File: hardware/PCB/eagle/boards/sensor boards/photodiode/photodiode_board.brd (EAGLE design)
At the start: 14.9 x 12.7 mm, 5 parts

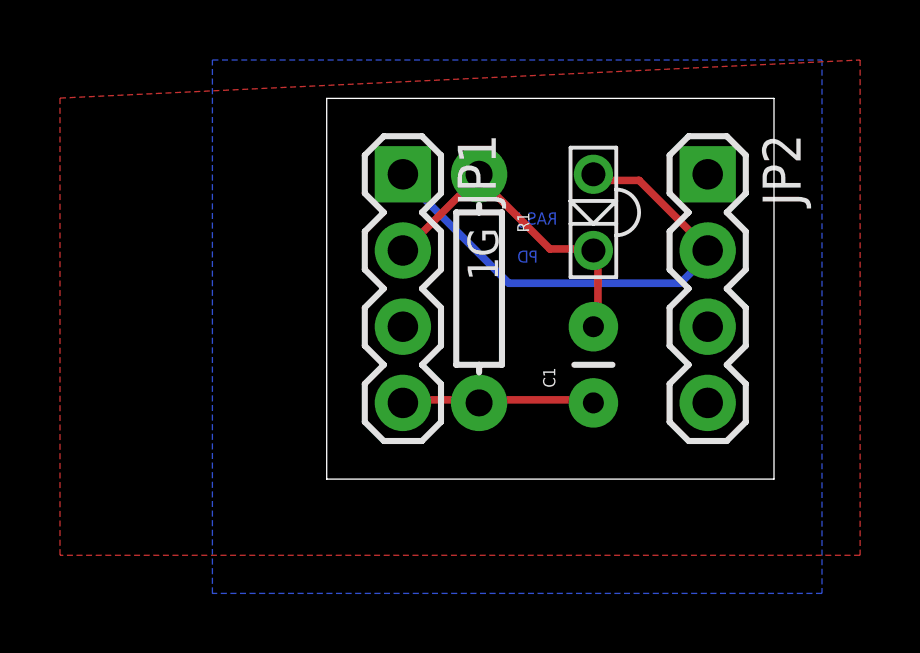
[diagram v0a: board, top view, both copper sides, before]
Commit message: updated
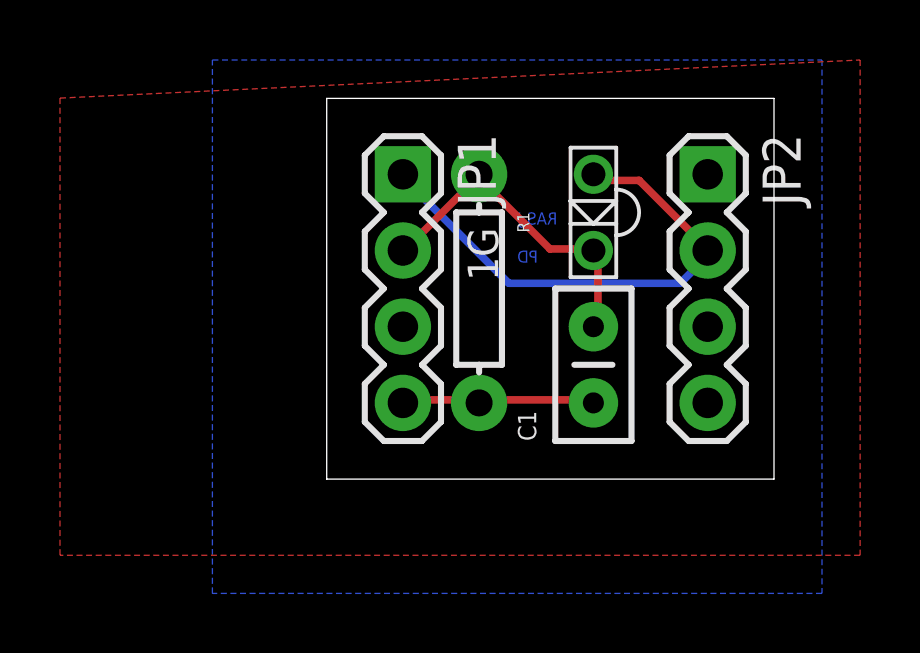
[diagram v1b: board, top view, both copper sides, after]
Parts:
- C1: device SparkFun-Capacitors:CAP-PTH-SMALL -> passive_components:TH_0.1-CAP
- D2: device SparkFun-LED:LTE-302 -> passive_components:TH_0.1-PD
- JP1, JP2: device SparkFun-Connectors:1X04 -> passive_components:1X04
- R1: device SparkFun-Resistors:AXIAL-0.3 -> passive_components:TH_0.3-RES
- moved JP1 3.81 mm to (2.54, 6.35)
- moved JP2 3.81 mm to (12.7, 6.35)
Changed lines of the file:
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@@
 <setting verticaltext="up"/>
 </settings>
-<grid distance="0.05" unitdist="inch" unit="inch" style="lines" multiple="1" display="yes" altdistance="0.025" altunitdist="inch" altunit="inch"/>
+<grid distance="0.05" unitdist="inch" unit="mm" style="lines" multiple="1" display="yes" altdistance="0.025" altunitdist="inch" altunit="inch"/>
 <layers>
 <layer number="1" name="Top" color="4" fill="1" visible="yes" active="yes"/>
@@
 <layer number="220" name="220bmp" color="21" fill="1" visible="no" active="no"/>
 <layer number="221" name="221bmp" color="22" fill="1" visible="no" active="no"/>
-<layer number="222" name="222bmp" color="23" fill="1" visible="no" active="no"/>
 <layer number="223" name="223bmp" color="24" fill="1" visible="no" active="no"/>
 <layer number="224" name="224bmp" color="25" fill="1" visible="no" active="no"/>
@@
 </autorouter>
 <elements>
-<element name="C1" library="SparkFun-Capacitors" package="CAP-PTH-SMALL" value="" x="8.89" y="2.54" rot="R90"/>
-<element name="D2" library="SparkFun-LED" package="LTE-302" value="PD" x="8.89" y="8.89" rot="R90"/>
-<element name="JP1" library="SparkFun-Connectors" package="1X04" value="" x="2.54" y="10.16" rot="R270"/>
-<element name="JP2" library="SparkFun-Connectors" package="1X04" value="" x="12.7" y="10.16" rot="R270"/>
-<element name="R1" library="SparkFun-Resistors" package="AXIAL-0.3" value="1G" x="5.08" y="6.35" rot="R270"/>
+<element name="C1" library="passive_components" package="TH_0.1-CAP" value="" x="8.89" y="2.54" rot="R90"/>
+<element name="D2" library="passive_components" package="TH_0.1-PD" value="PD" x="8.89" y="8.89" rot="R90"/>
+<element name="JP1" library="passive_components" package="1X04" value="" x="2.54" y="6.35" rot="R270"/>
+<element name="JP2" library="passive_components" package="1X04" value="" x="12.7" y="6.35" rot="R270"/>
+<element name="R1" library="passive_components" package="TH_0.3-RES" value="1G" x="5.08" y="6.35" rot="R270"/>
 </elements>
 <signals>
